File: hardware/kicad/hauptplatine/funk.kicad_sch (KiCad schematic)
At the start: 17 parts, among them U401 Ra-01SH, U402 64 Mbit SOIC-8 208 mil

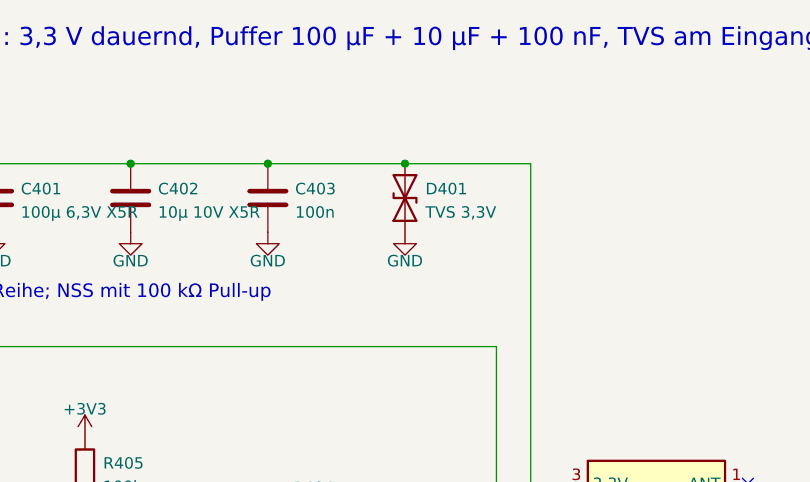
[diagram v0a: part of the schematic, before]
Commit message: update
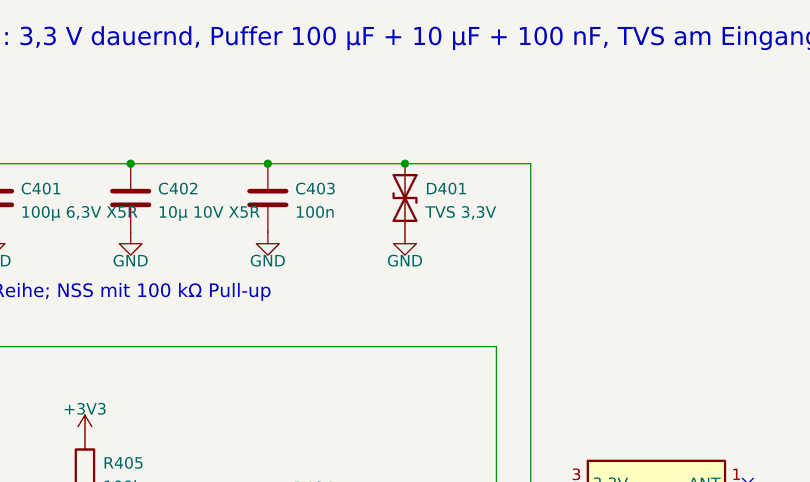
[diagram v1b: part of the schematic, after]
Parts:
- U401: footprint (none) -> Bienen:Ai-Thinker_Ra-01SH
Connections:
- net +3V3: now also D401.1 (A1); no longer D401.2 (A2)
- net GND: now also D401.2 (A2); no longer D401.1 (A1)
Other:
- moved on the sheet: D401
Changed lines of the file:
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@@
 			)
 		)
-		(property "Footprint" ""
+		(property "Footprint" "Bienen:Ai-Thinker_Ra-01SH"
 			(at 190.5 127 0)
 			(hide yes)
@@
 	(symbol
 		(lib_id "Device:D_TVS")
-		(at 162.56 82.55 90)
+		(at 162.56 82.55 270)
 		(unit 1)
 		(body_style 1)
@@
 					(size 1.27 1.27)
 				)
-				(justify right)
+				(justify left)
 			)
 		)
@@
 					(size 1.27 1.27)
 				)
-				(justify right)
+				(justify left)
 			)
 		)
@@
 			)
 		)
-		(property "Description" "ESD-Schutz am 3,3-V-Eingang des Moduls (Datenblatt-Empfehlung); Teil wählen [P]"
+		(property "Description" "ESD-Schutz am 3,3-V-Eingang des Moduls (Datenblatt-Empfehlung); Pad 1 an +3V3, damit auch eine unidirektionale TVS (Kathode = Pad 1) richtig sitzt; Teil wählen [P]"
 			(at 162.56 82.55 0)
 			(hide yes)

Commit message: update
"Hauptplatine grob platziert (platine_bestuecken.py, 139 Bauteile, Schaltplanabgleich 0); Gehäuse mit STEP geprüft: Lochbild bestätigt, Freiraum über Platine >= 44,3 mm (HW-03 erfüllt), Dombohrung Ø 2,4 mm korrigiert, Lichtleiter ca. 19,4 mm. Tests: ERC 0, Netzprüfung 178/178, alle_tests_linux.sh rc=0"
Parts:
- JP401, JP402: now left out of the parts list
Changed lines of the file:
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@@
 		(body_style 1)
 		(exclude_from_sim no)
-		(in_bom yes)
+		(in_bom no)
 		(on_board yes)
 		(in_pos_files yes)
@@
 		(body_style 1)
 		(exclude_from_sim no)
-		(in_bom yes)
-		(on_board yes)
-		(in_pos_files yes)
+		(in_bom no)
+		(on_board yes)
+		(in_pos_files yes)
